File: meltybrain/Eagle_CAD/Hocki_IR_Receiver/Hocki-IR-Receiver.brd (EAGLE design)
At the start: 42 x 34 mm, 69 parts, among them U1 OPA2380AIDGKR, U10 LMH6612MAX/NOPB, U11 LMH6612MAX/NOPB, U2 OPA2380AIDGKR, U3 TLV3502AIDCNR, U4 TLV3502AIDCNR, U5 SN74LVC1G58DCKR, U6 NL27WZ32USG, U7 TMUX1204DGSR, U8 LP38693MP-5.0/NOPB, U9 TLV73310PDBVT

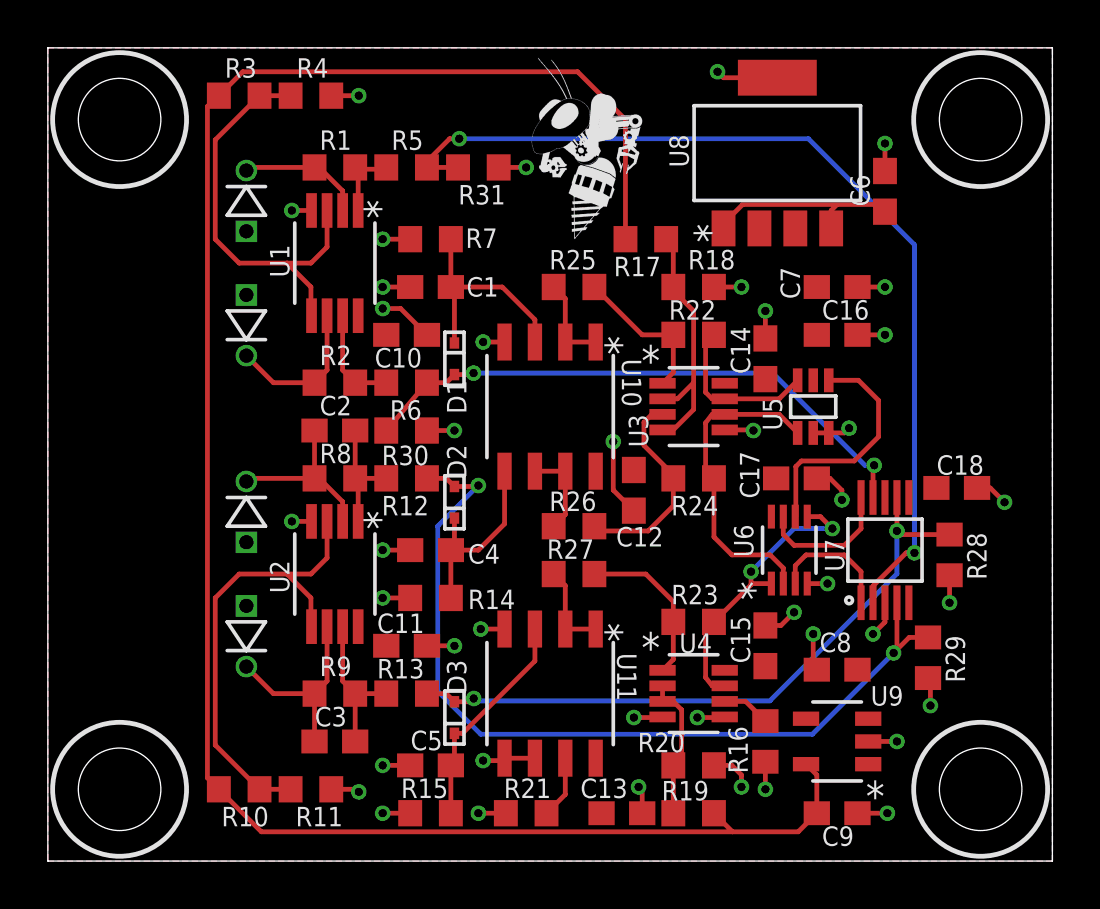
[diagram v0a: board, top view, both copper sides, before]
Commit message: progress...
IR receiver has all parts accounting BoM
started doing that for control
progress on control layout
Varun I hate this...
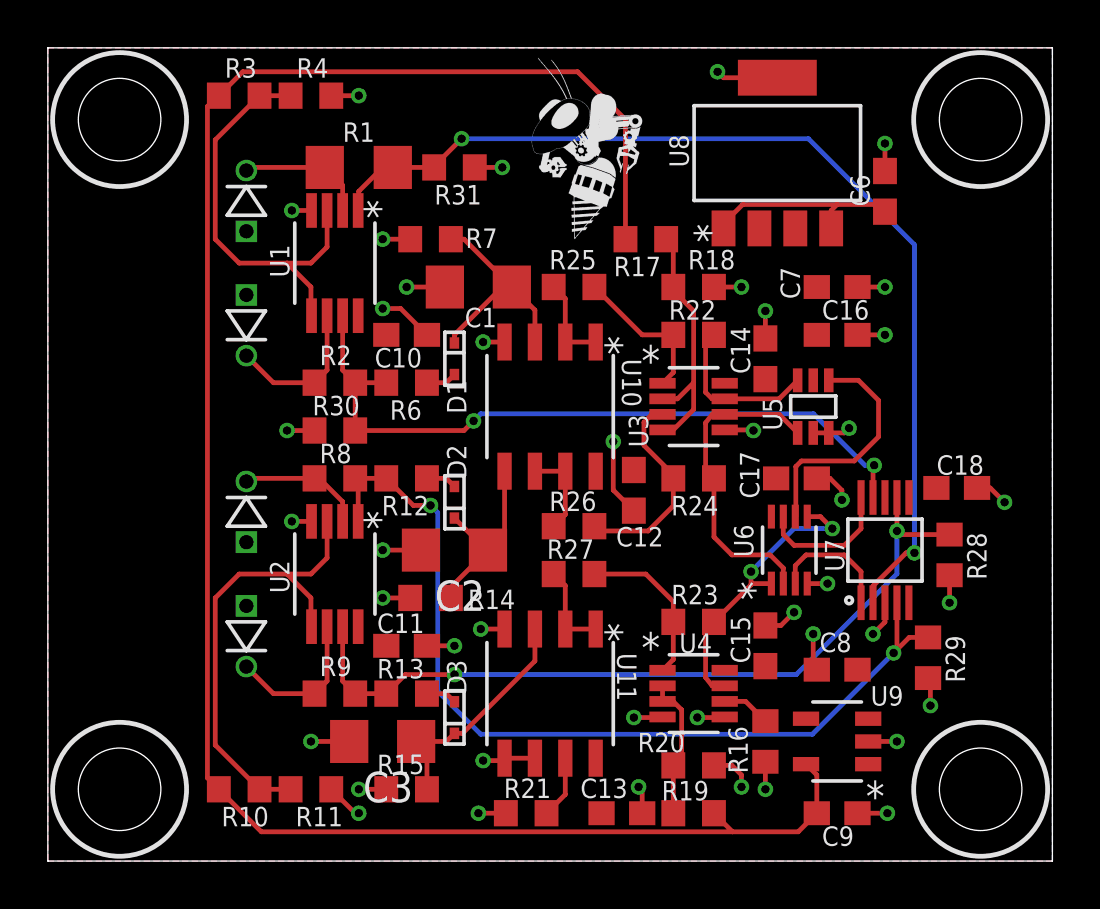
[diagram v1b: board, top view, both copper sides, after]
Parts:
- removed C4, C5: 50n, rcl:C0603
- removed R5: 50, resistor:R0603
- C1: value 50n -> 47n; device rcl:C0603 -> rcl:C1206
- C2: value 0.5p -> 47n; device rcl:C0603 -> rcl:C1206
- C3: value 2p -> 47n; device rcl:C0603 -> rcl:C1206
- R1: device resistor:R0603 -> rcl:R1206
- R10, R11, R16, R21, R28, R29, R3, R30, R31, R4: value 500 -> 499
- R14, R15, R7: value 30k -> 31.6k
- moved C2 7.07 mm to (17.0, 13.0), turned to 180 degrees
- moved R30 3.00 mm to (12.0, 18.0), turned to 0 degrees
- moved C1 2.00 mm to (18.0, 24.0)
- moved C3 2.00 mm to (14.0, 5.00), turned to 180 degrees
- moved R15 1.41 mm to (15.0, 3.00)
- moved R1 1.00 mm to (13.0, 29.0)
- moved R31 1.00 mm to (17.0, 29.0)
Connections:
- removed net N$11: C3.2, R13.1, R9.2, U2.7
- removed net N$8: C2.2, R12.1, R8.2, U2.1
- new net N$21: D1.2, R6.2
- net 100KGAIN: now also R12.1, R8.2, U2.1; no longer D2.2, R12.2
- net 100KPEAK: now also C2.1; no longer C4.1
- net 10KGAIN: now also R13.1, R9.2, U2.7; no longer D3.2, R13.2
- net 10KPEAK: now also C3.1; no longer C5.1
- net 10MGAIN: now also R1.2, U1.1; no longer R5.2
- net 1MGAIN: now also R2.2, R6.1, U1.7; no longer D1.2, R6.2
- net GND: now also C2.2, C3.2; no longer C4.2, C5.2
- net N$10: no longer C3.1
- net N$2: now also D2.2, R12.2; no longer R1.2, R5.1, U1.1
- net N$4: now also D3.2, R13.2; no longer R2.2, R6.1, U1.7
- net N$6: no longer C2.1
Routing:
- net N$11: track 6.32 -> 0.00 mm
- net 1MGAIN: track 24.5 -> 30.6 mm
- net 10KGAIN: track 27.5 -> 33.2 mm
- net N$8: track 5.15 -> 0.00 mm
- net N$4: track 4.32 -> 1.29 mm
- net 10MGAIN: track 40.4 -> 42.7 mm
- net N$10: track 8.34 -> 6.34 mm
- net N$6: track 7.31 -> 5.31 mm
- net N$2: track 3.11 -> 1.29 mm
- net 100KGAIN: track 36.7 -> 38.4 mm
- net GND: track 56.0 -> 57.7 mm
- net N$21: track 0.00 -> 1.29 mm
- net 10KPEAK: track 9.36 -> 9.88 mm
